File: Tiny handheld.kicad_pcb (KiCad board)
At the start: 2 copper layers, 34.3 x 58.4 mm, 42 parts, among them J1 Conn_01x04_Female, J3 TYPE-C-31-M-12, U1 ATtiny85-20P, U2 ATtiny85-20M, U3 EEPROM-I2CEIAJ

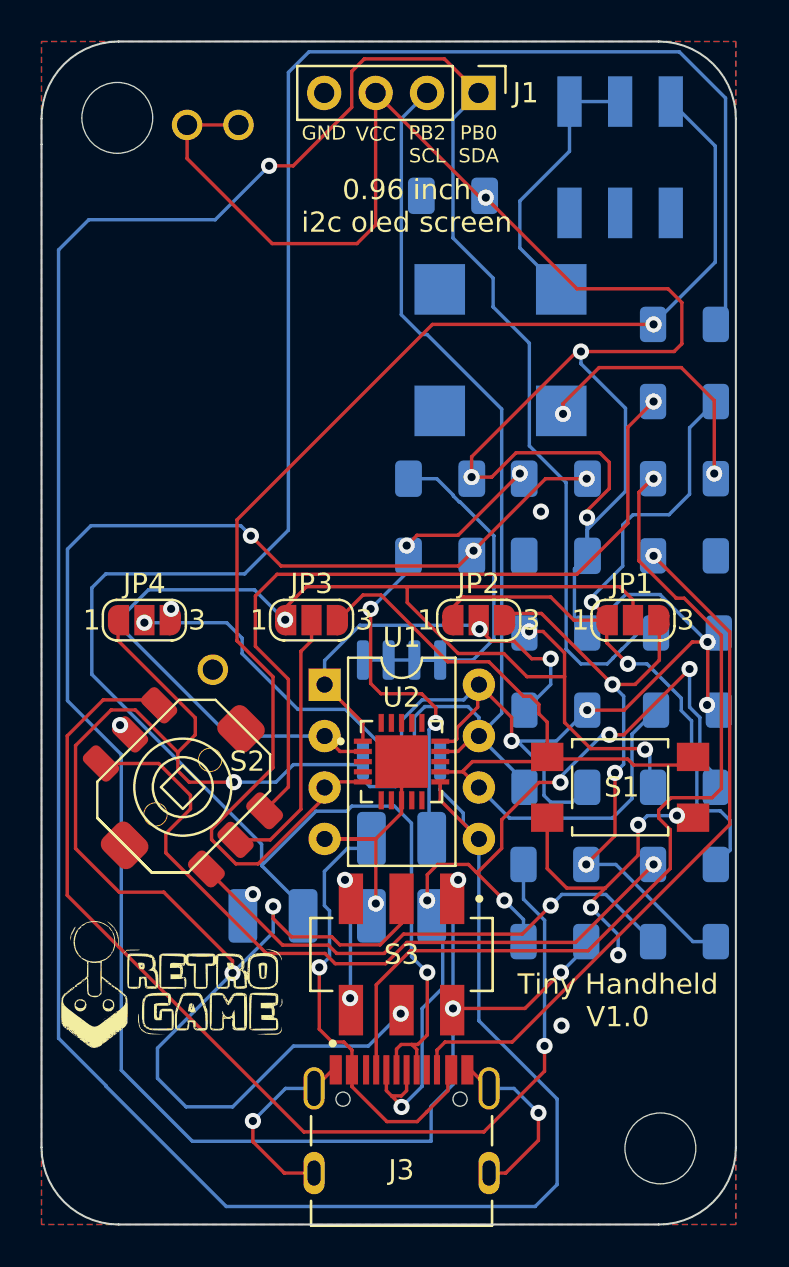
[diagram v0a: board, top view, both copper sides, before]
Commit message: Added curvy wires
Because they are the best thing in this straight world
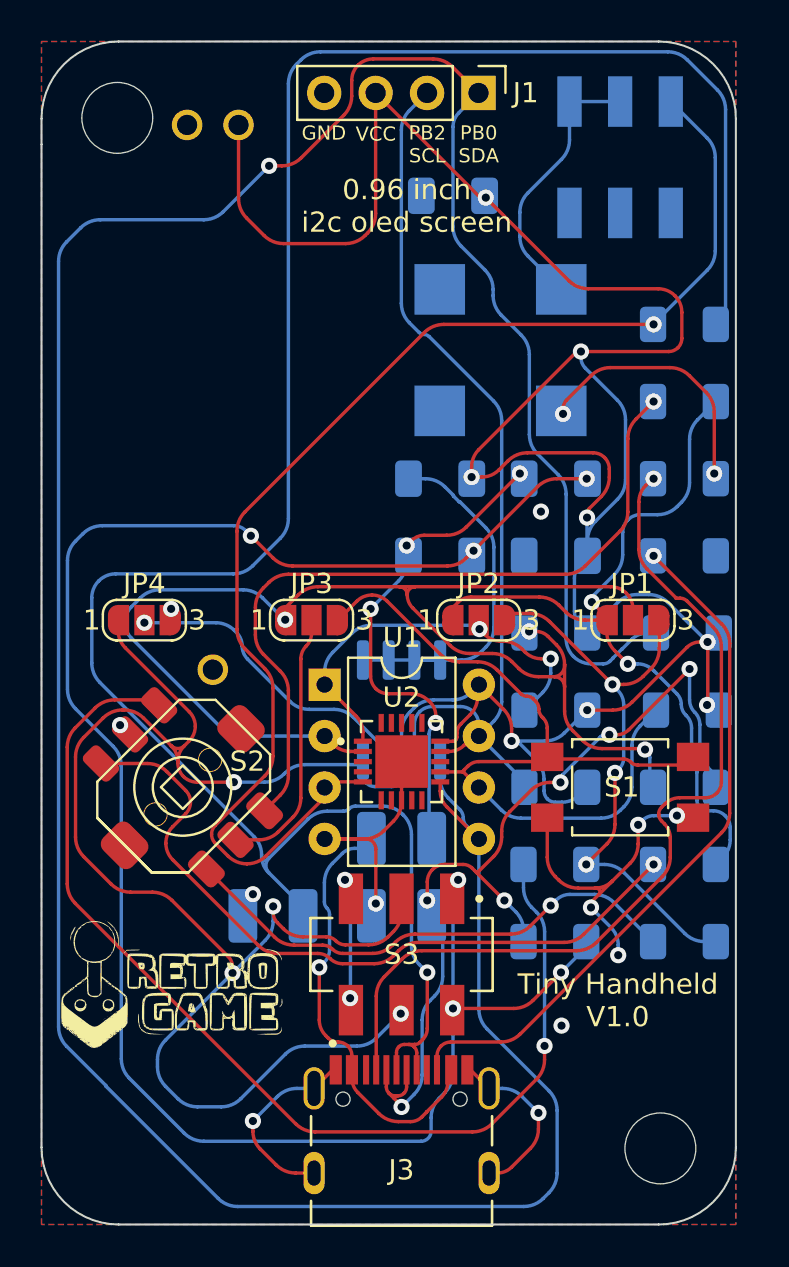
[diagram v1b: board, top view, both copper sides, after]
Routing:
- net VCC: track 208.4 -> 201.9 mm
- net PB0/SDA/MOSI: track 155.5 -> 153.8 mm
- net Net-(JP1-Pad1): track 38.8 -> 37.5 mm
- net ExtVCC: track 93.6 -> 92.5 mm
- net PB3: track 64.9 -> 65.8 mm
- net PB4: track 65.5 -> 64.8 mm
- net Net-(J3-PadA5): track 45.3 -> 44.6 mm
- net PB1/MISO: track 42.2 -> 41.5 mm
- net GND: track 78.5 -> 77.8 mm
- net Net-(R7-Pad2): track 36.8 -> 36.2 mm
- net Net-(D1-Pad2): track 21.2 -> 20.7 mm
- net Net-(R1-Pad2): track 53.2 -> 52.7 mm
- net Net-(R4-Pad2): track 38.2 -> 37.7 mm
